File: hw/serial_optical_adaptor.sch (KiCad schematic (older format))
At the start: 11 parts, among them P1 USB_OTG, U1 LM393

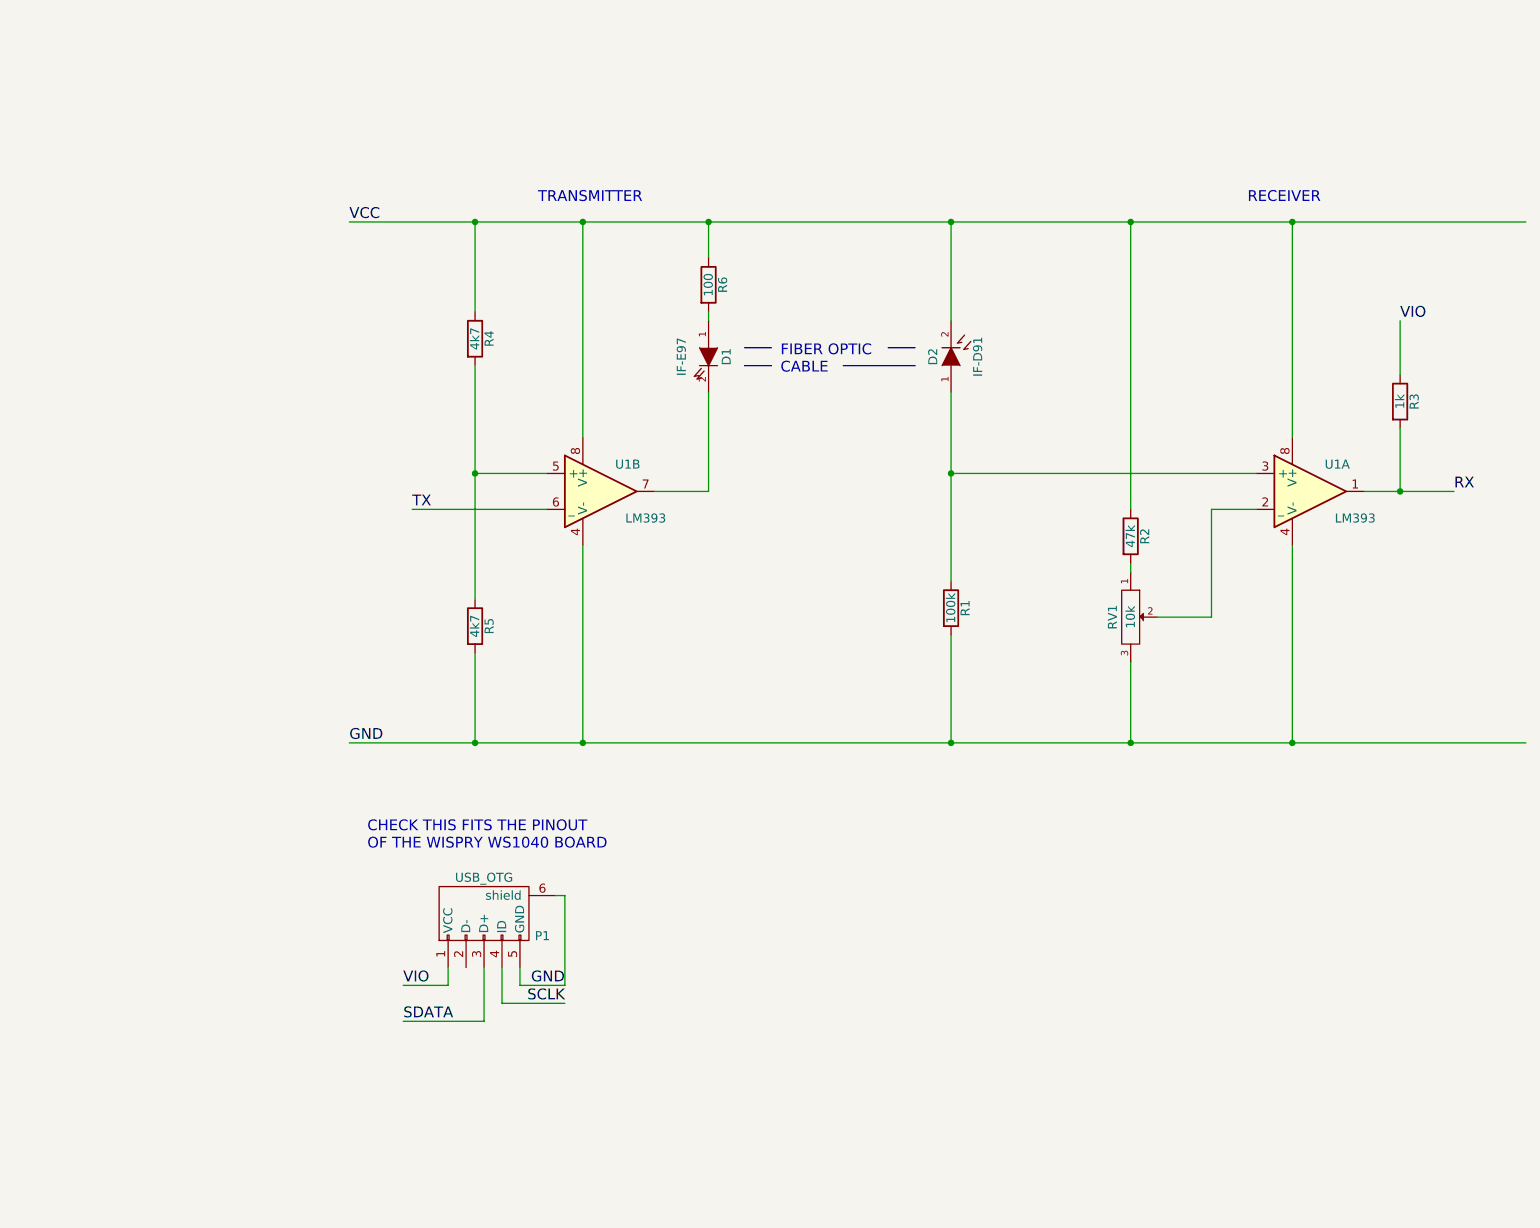
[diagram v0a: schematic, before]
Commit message: A    hw/SMTU2032-1.kicad_mod A    hw/adg3300.dcm A    hw/lp3984.dcm A    hw/lp3984.lib M    hw/serial_optical_adaptor-cache.lib M    hw/serial_optical_adaptor.bak M    hw/serial_optical_adaptor.pro M    hw/serial_optical_adaptor.sch
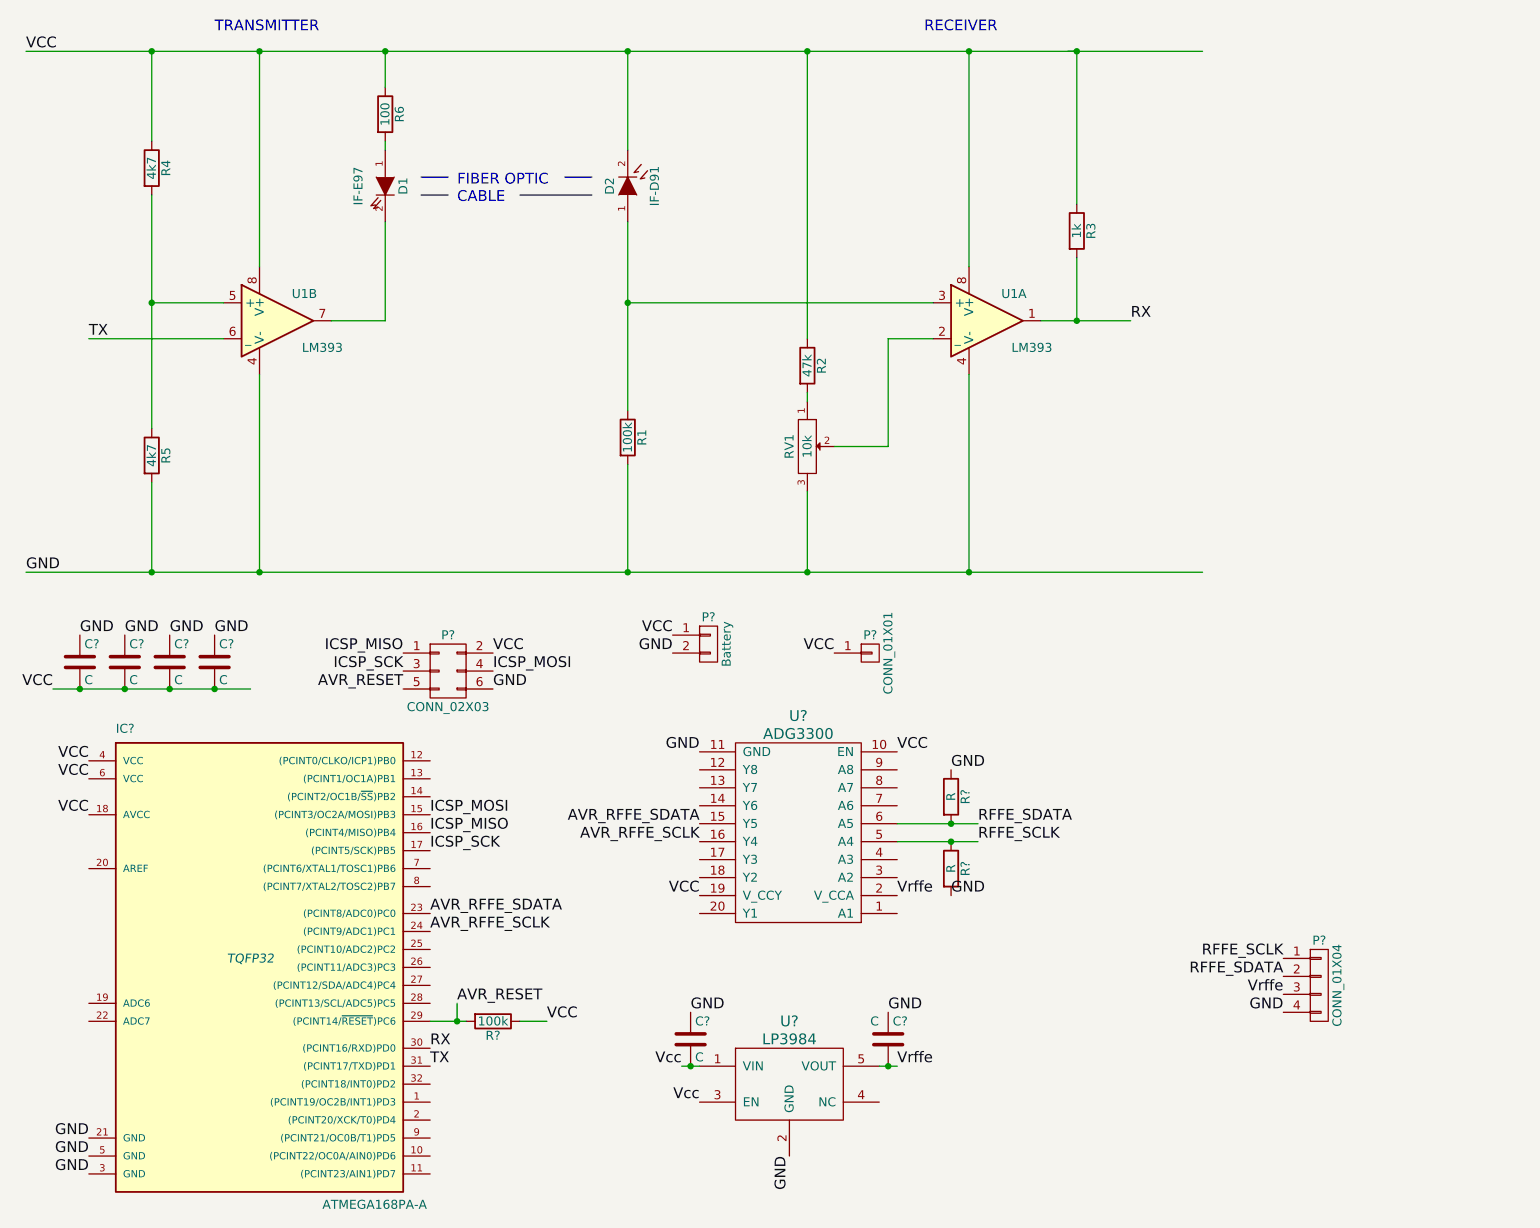
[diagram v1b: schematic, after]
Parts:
- removed P1: USB_OTG, kicadlib:smd_amphenol_usb_micro-b, symbol USB_OTG
- added C? (x6): C, symbol C
- added IC?: ATMEGA168PA-A, TQFP32, symbol ATMEGA168PA-A
- added P?: CONN_02X03, symbol CONN_02X03
- added P?: CONN_01X01, symbol CONN_01X01
- added P?: CONN_01X04, symbol CONN_01X04
- added P?: Battery, symbol CONN_01X02
- added R?: 100k, symbol R
- added R? (x2): R, symbol R
- added U?: ADG3300, symbol ADG3300
- added U?: LP3984, symbol LP3984
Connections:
- net labels added: AVR_RESET, AVR_RFFE_SCLK, AVR_RFFE_SDATA, ICSP_MISO, ICSP_MOSI, ICSP_SCK, RFFE_SCLK, RFFE_SDATA, Vcc, Vrffe
- net labels removed: SCLK, SDATA, VIO
- wire segments 38 -> 37
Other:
- note removed: "CHECK THIS FITS THE PINOUT\nOF THE WISPRY WS1040 BOARD"
- moved on the sheet: D1, D2, R1, R2, R3, R4, R5, R6, RV1, U1A, U1B
